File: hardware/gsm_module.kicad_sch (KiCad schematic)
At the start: 30 parts, among them IC2 DALC208SC6, J6 JAE_SIM_Card_SF72S006

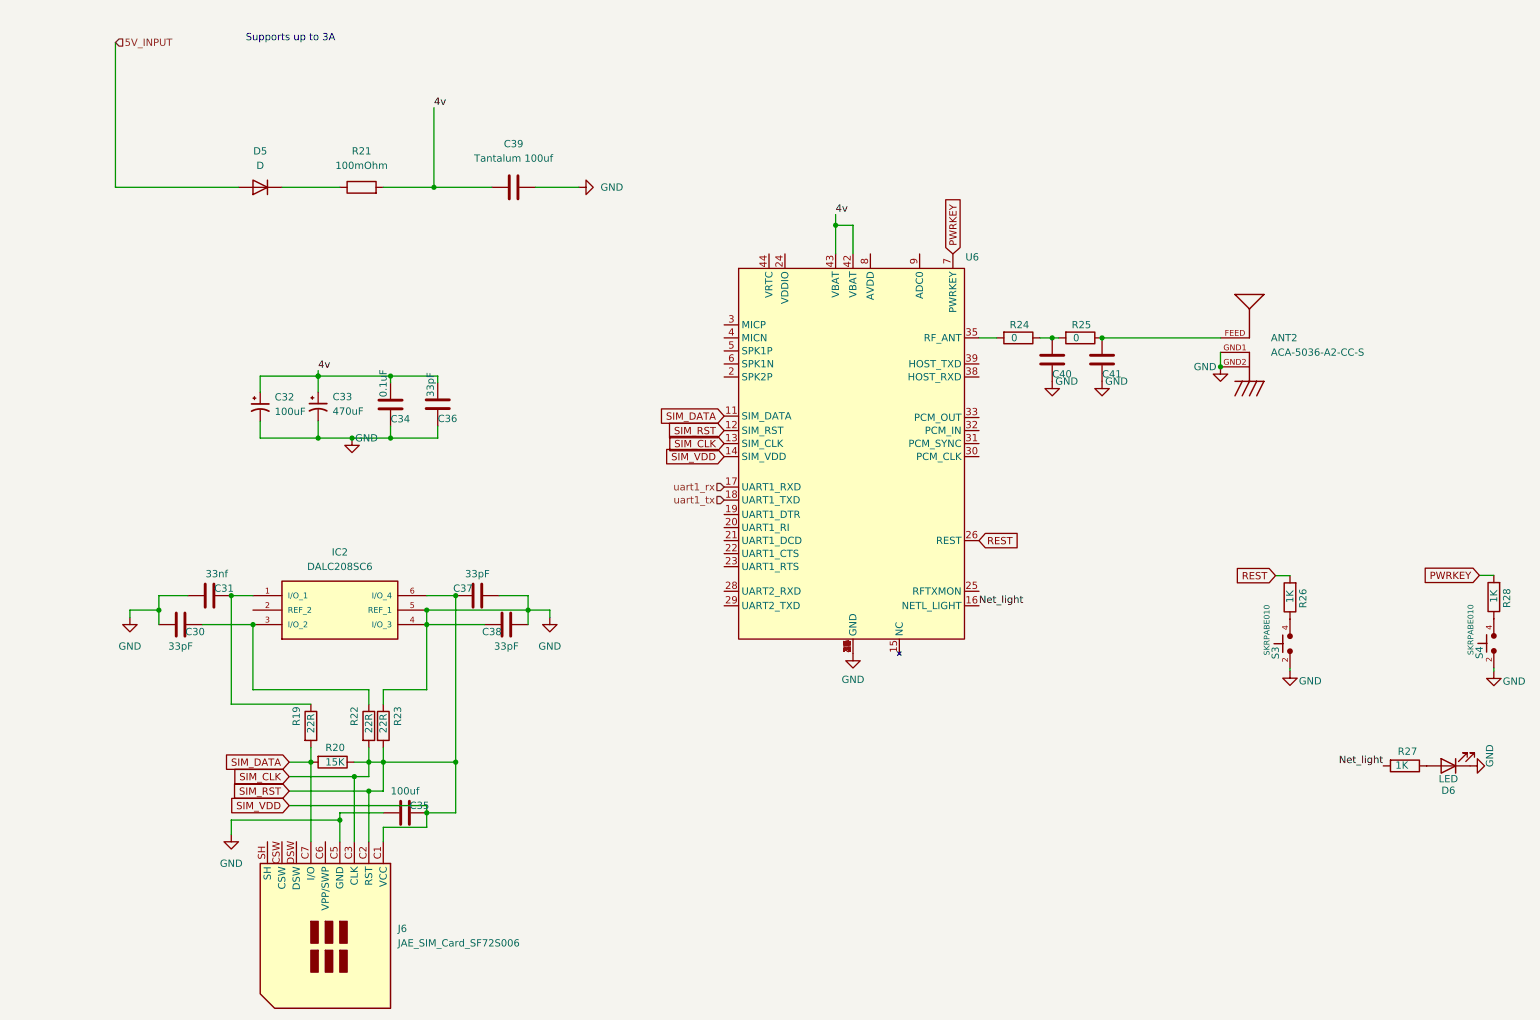
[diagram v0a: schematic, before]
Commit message: Kicad şema düzenlemesi yapıldı.
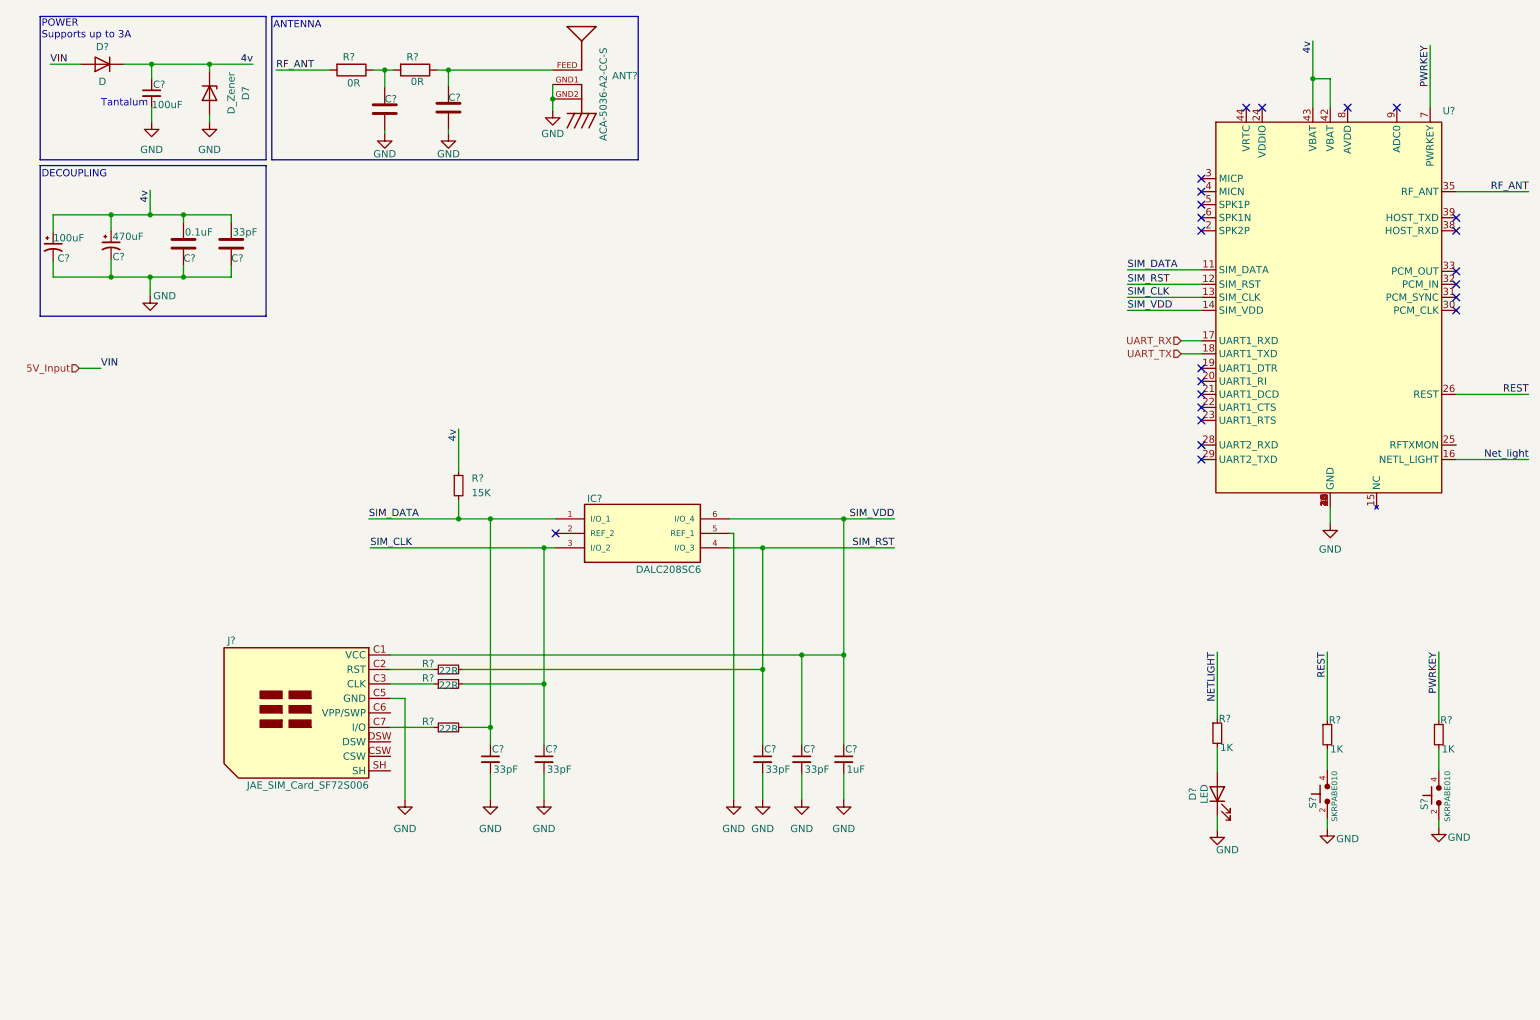
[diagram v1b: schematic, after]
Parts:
- removed ANT2: ACA-5036-A2-CC-S, mergened_footprints:ACA-5036-A2-CC-S, symbol mergened_symbols:ACA-5036-A2-CC-S
- removed C30, C36, C37, C38: 33pF, Capacitor_SMD:C_0805_2012Metric, symbol Device:C
- removed C31: 33nf, Capacitor_SMD:C_0805_2012Metric, symbol Device:C
- removed C32: 100uF, Capacitor_SMD:CP_Elec_8x10.5, symbol Device:C_Polarized_Small_US
- removed C33: 470uF, Capacitor_SMD:CP_Elec_8x10.5, symbol Device:C_Polarized_Small_US
- removed C34: 0.1uF, Capacitor_SMD:C_0805_2012Metric, symbol Device:C
- removed C35: 100uf, drip-irrigation-sys-cc:CAP_WCAP-ASLI_06p3X05p5_WRE, symbol Device:C
- removed C39: Tantalum 100uf, Capacitor_Tantalum_SMD:CP_EIA-6032-20_AVX-F, symbol Device:C
- removed C40, C41: ~, Capacitor_SMD:C_0805_2012Metric, symbol Device:C
- removed D5: D, drip-irrigation-sys-cc:DO-201AD_STM, symbol Device:D
- removed D6: LED, LED_SMD:LED_0805_2012Metric, symbol Device:LED
- removed IC2: DALC208SC6, mergened_footprints:DALC208SC6, symbol DALC208SC6:DALC208SC6
- removed J6: JAE_SIM_Card_SF72S006, Connector_JAE:JAE_SIM_Card_SF72S006, symbol Connector:JAE_SIM_Card_SF72S006
- removed R19, R22, R23: 22R, Resistor_SMD:R_0603_1608Metric, symbol Device:R
- removed R20: 15K, Resistor_SMD:R_0603_1608Metric, symbol Device:R
- removed R21: 100mOhm, Resistor_SMD:R_2512_6332Metric, symbol Device:R
- removed R24, R25: 0, Resistor_SMD:R_0603_1608Metric, symbol Device:R
- removed R26, R27, R28: 1K, Resistor_SMD:R_0603_1608Metric, symbol Device:R
- removed S3, S4: SKRPABE010, symbol Button_SKRPABE010:SKRPABE010
- removed U6: ~, mergened_footprints:MG2608, symbol mergened_symbols:mg2608
- added ANT?: ACA-5036-A2-CC-S, drip-irrigation-sys-cc:ACA-5036-A2-CC-S, symbol mergened_symbols:ACA-5036-A2-CC-S
- added C?: 470uF, Capacitor_SMD:CP_Elec_8x10.5, symbol Device:C_Polarized_Small_US
- added C?: 0.1uF, Capacitor_SMD:C_0805_2012Metric, symbol Device:C
- added C? (x4): 33pF, Capacitor_SMD:C_0805_2012Metric, symbol Device:C_Small
- added C?: 100uF, Capacitor_SMD:CP_Elec_8x10.5, symbol Device:C_Polarized_Small_US
- added C? (x2): ~, Capacitor_SMD:C_0805_2012Metric, symbol Device:C
- added C?: 100uF, Capacitor_SMD:C_0805_2012Metric, symbol Device:C_Small
- added C?: 33pF, Capacitor_SMD:C_0805_2012Metric, symbol Device:C
- added C?: 1uF, Capacitor_SMD:C_0805_2012Metric, symbol Device:C_Small
- added D7: D_Zener, drip-irrigation-sys-cc:SMB-2_4P60X3P95_ONS, symbol Device:D_Zener
- added D?: D, Diode_SMD:D_SOD-123F, symbol Device:D
- added D?: LED, LED_SMD:LED_0805_2012Metric, symbol Device:LED
- added IC?: DALC208SC6, drip-irrigation-sys-cc:SOT23-6L_STM, symbol DALC208SC6:DALC208SC6
- added J?: JAE_SIM_Card_SF72S006, Connector_JAE:JAE_SIM_Card_SF72S006, symbol Connector:JAE_SIM_Card_SF72S006
- added R? (x3): 22R, Resistor_SMD:R_0603_1608Metric, symbol Device:R_Small
- added R? (x3): 1K, Resistor_SMD:R_0603_1608Metric, symbol Device:R_Small
- added R?: 15K, Resistor_SMD:R_0603_1608Metric, symbol Device:R_Small
- added R? (x2): 0R, Resistor_SMD:R_0603_1608Metric, symbol Device:R
- added S? (x2): SKRPABE010, drip-irrigation-sys-cc:SW_PTS636_CNK, symbol Button_SKRPABE010:SKRPABE010
- added U?: ~, drip-irrigation-sys-cc:MG2608, symbol mergened_symbols:mg2608
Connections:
- net 4v: now also C?.1, C?.1, C?.1, C?.1, C?.1, D7.1 (K), D?.1 (K), R?.1, U?.42 (VBAT), U?.43 (VBAT)
- net GND: now also ANT?.GND1, ANT?.GND2, C?.2, C?.2, C?.2, C?.2, C?.2, C?.2, C?.2, C?.2, C?.2, C?.2, C?.2, C?.2, D7.2 (A), D?.1 (K), IC?.5 (REF_1), J?.C5 (GND), S?., S?., S?.2, S?.2, U?.1 (GND), U?.10 (GND), U?.27 (GND), U?.34 (GND), U?.36 (GND), U?.37 (GND), U?.40 (GND), U?.41 (GND)
- net Net_light: now also U?.16 (NETL_LIGHT)
- net PWRKEY: now also R?.1, U?.7 (PWRKEY)
- net REST: now also R?.1, U?.26 (REST)
- net SIM_CLK: now also C?.1, IC?.3 (I/O_2), R?.2, U?.13 (SIM_CLK)
- net SIM_DATA: now also C?.1, IC?.1 (I/O_1), R?.2, R?.2, U?.11 (SIM_DATA)
- new net: ANT?.FEED, C?.1, R?.1
- new net: J?.C2 (RST), R?.1
- new net: D?.2 (A), R?.2
- new net: J?.C3 (CLK), R?.1
- new net: J?.C7 (I/O), R?.1
- new net: R?.2, S?., S?.4 (x2)
- new net: C?.1, R?.1, R?.2
- new net 5V_Input: D?.2 (A)
- new net NETLIGHT: R?.1
- new net RF_ANT: R?.2, U?.35 (RF_ANT)
- new net SIM_RST: C?.1, IC?.4 (I/O_3), R?.2, U?.12 (SIM_RST)
- new net SIM_VDD: C?.1, C?.1, IC?.6 (I/O_4), J?.C1 (VCC), U?.14 (SIM_VDD)
- new net UART_RX: U?.17 (UART1_RXD)
- new net UART_TX: U?.18 (UART1_TXD)
- no-connect marks 0 -> 23
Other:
- note added: "ANTENNA"
- note added: "DECOUPLING"
- note added: "POWER Supports up to 3A"
- note added: "Tantalum"
- note removed: "Supports up to 3A"
